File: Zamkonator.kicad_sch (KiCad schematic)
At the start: 27 parts, among them J1 Screw_Terminal_01x06, J3 Conn_01x08_Male, J4 Conn_02x06_Counter_Clockwise, J5 Conn_01x04_Female, J6 Conn_01x03_Female

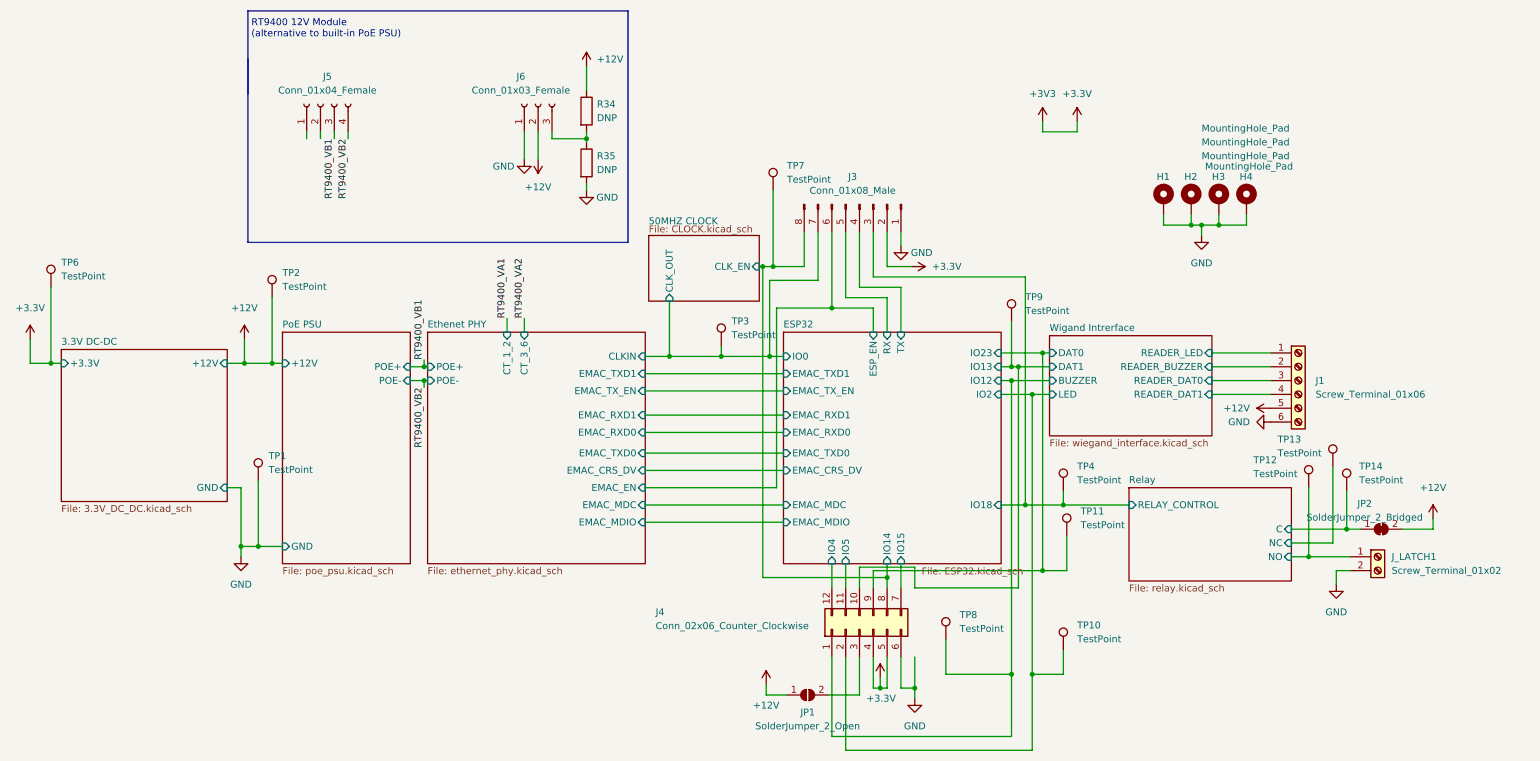
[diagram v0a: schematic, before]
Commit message: Update kicad files
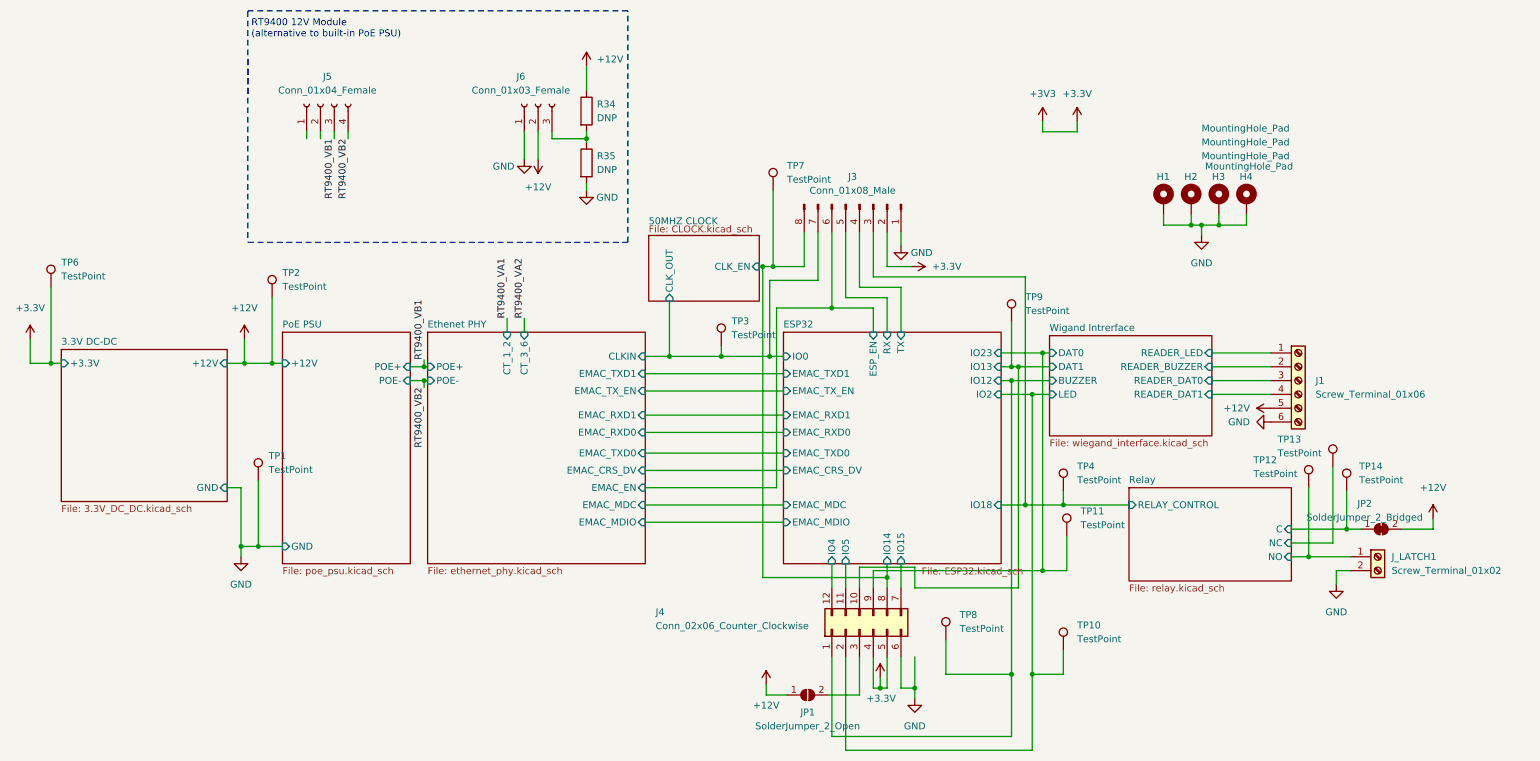
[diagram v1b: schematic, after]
